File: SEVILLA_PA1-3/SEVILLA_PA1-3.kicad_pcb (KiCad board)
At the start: 2 copper layers, 100 x 50 mm, 14 parts, among them SW3 SW_SPST, SW4 SW_SPST, U1 HDSP-7401, U2 PIC16F84A-XXP, U3 HDSP-7401, Y1 4 MHz

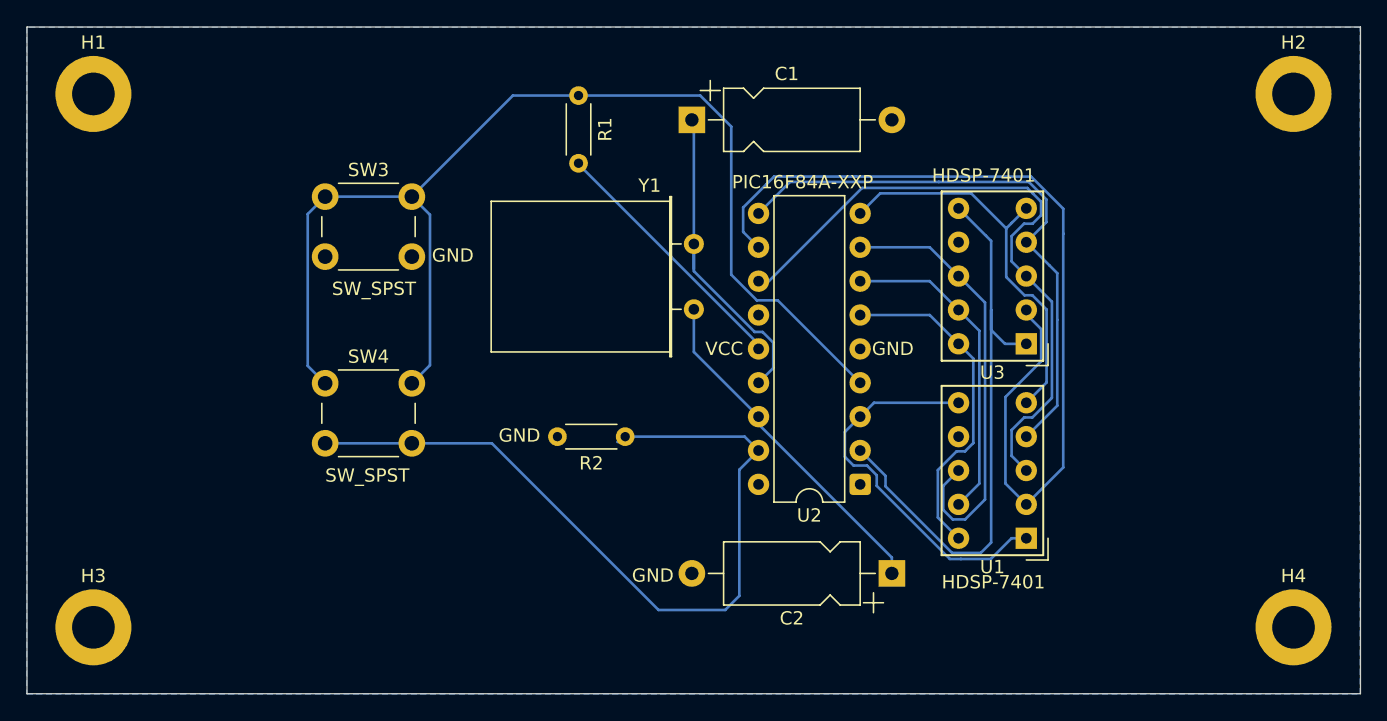
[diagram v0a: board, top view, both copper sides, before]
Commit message: Refactor code structure and remove redundant sections for improved readability and maintainability
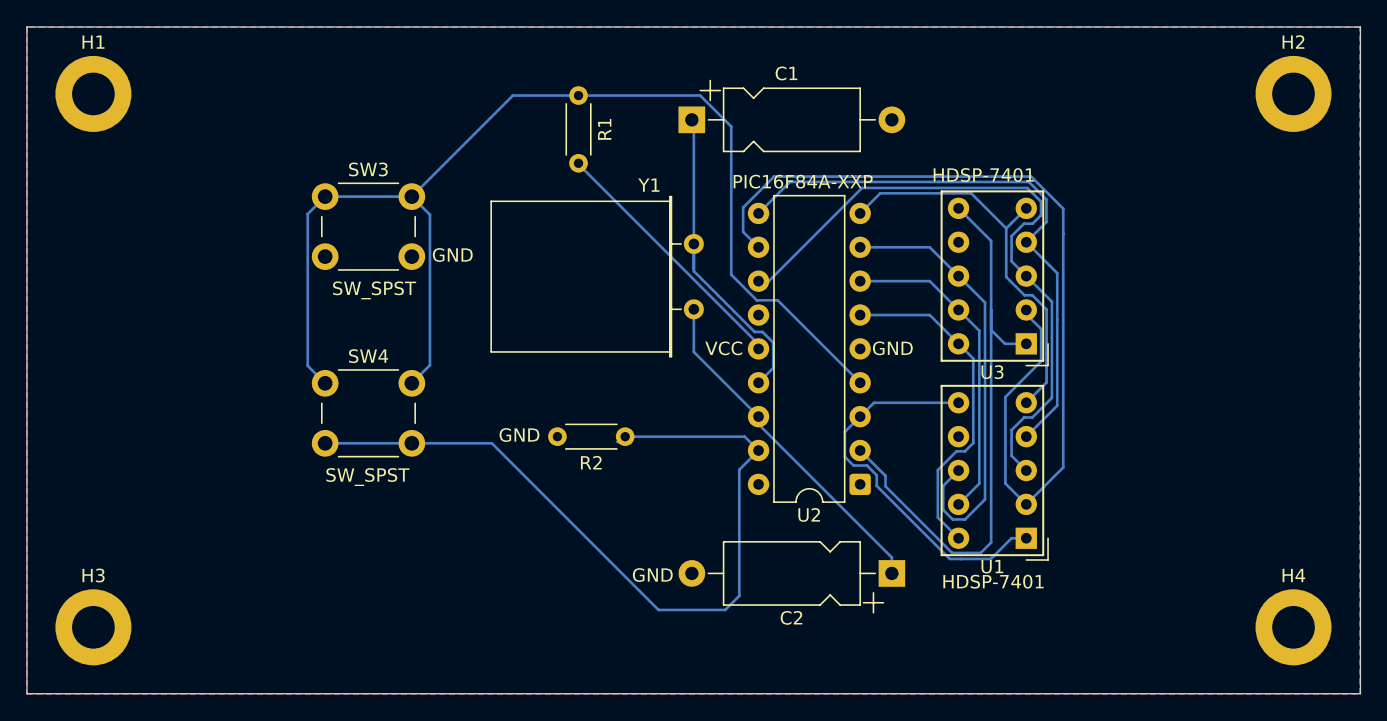
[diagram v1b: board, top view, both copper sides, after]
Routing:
- added copper zone on F.Cu, net GND
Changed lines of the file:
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@@
 		(net 1)
 		(net_name "GND")
-		(layer "B.Cu")
+		(layers "F.Cu" "B.Cu")
 		(hatch edge 0.5)
 		(connect_pads

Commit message: Refactor code structure and remove redundant sections for improved readability and maintainability
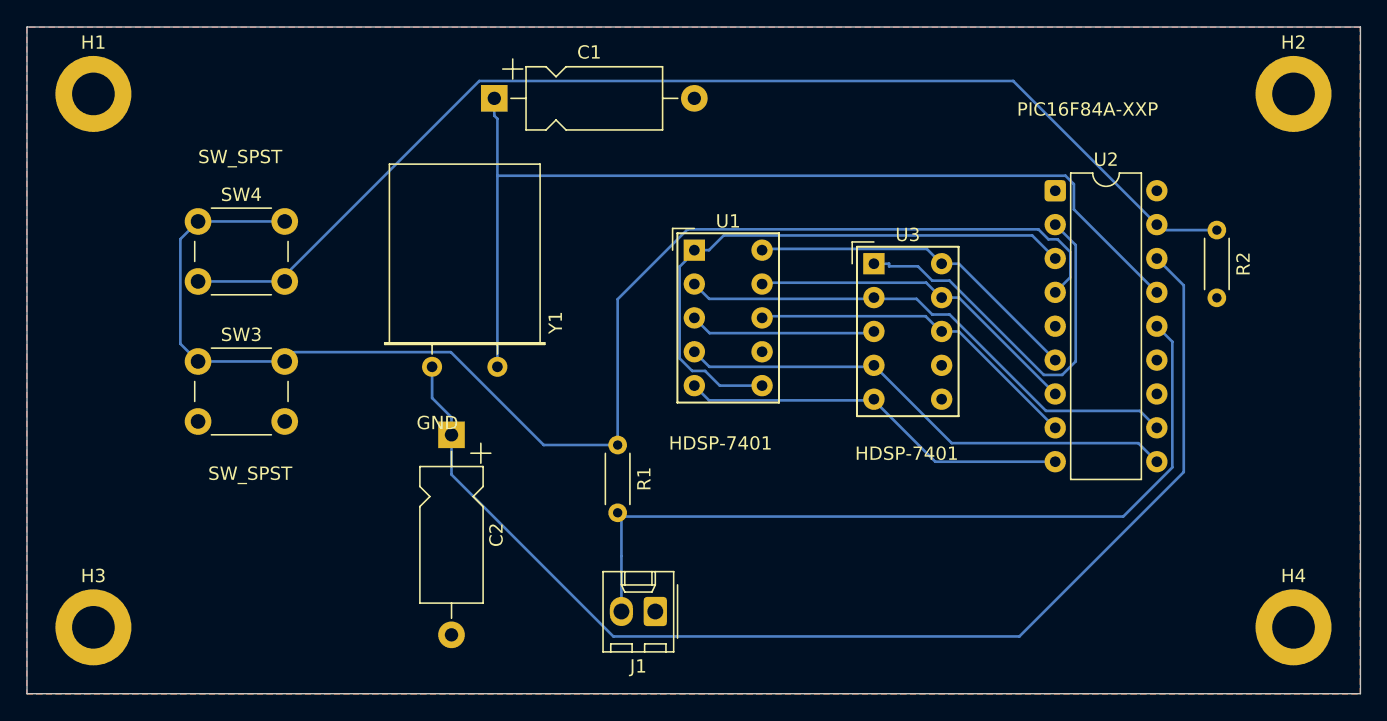
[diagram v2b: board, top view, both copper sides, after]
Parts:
- added J1: Conn_01x02, Connector_Molex:Molex_KK-254_AE-6410-02A_1x02_P2.54mm_Vertical, F.Cu at (143.6, 112.8)
- moved R2 47.0 mm to (185.8, 84.2), turned to -90 degrees
- moved C2 34.6 mm to (128.4, 99.6), turned to -90 degrees
- moved U1 33.0 mm to (146.6, 85.7), turned to 0 degrees
- moved U2 26.4 mm to (173.6, 81.3), turned to 0 degrees
- moved R1 26.4 mm to (140.8, 105.4)
- moved Y1 17.4 mm to (131.8, 94.5), turned to 180 degrees
- moved SW3 15.6 mm to (109.3, 94.1)
- moved SW4 15.4 mm to (109.3, 83.6)
- moved C1 14.9 mm to (131.6, 74.3)
- moved U3 12.9 mm to (160.0, 86.7), turned to 0 degrees
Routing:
- net Net-(U2-OSC1/CLKIN): track 26.0 -> 90.6 mm
- net Net-(U2-OSC2/CLKOUT): track 24.7 -> 74.4 mm
- net VCC: track 19.5 -> 61.4 mm
- net Net-(U1-G): track 49.3 -> 14.0 mm
- net Net-(U1-F): track 69.5 -> 39.2 mm
- net Net-(SW4-B): track 59.4 -> 87.5 mm
- net Net-(SW3-A): track 88.9 -> 104.0 mm
- net Net-(U2-TOCKI/RA4): track 29.2 -> 43.9 mm
- net Net-(U2-RA3): track 44.4 -> 30.0 mm
- net Net-(U1-C): track 33.3 -> 25.5 mm
- net Net-(U1-E): track 43.4 -> 38.2 mm
- net Net-(U1-B): track 24.1 -> 25.5 mm
- net Net-(U1-D): track 30.1 -> 29.5 mm
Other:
- board text removed: "VCC"
